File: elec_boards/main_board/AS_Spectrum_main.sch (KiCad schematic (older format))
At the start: 55 parts, among them J1 MODE, J10 Morpho_Gauche, J11 RN42X-DROITE, J12 POW-5V, J13 Bande1, J14 Morpho_Droite, J15 Lidar, J16 Bande2, J17 Bande3, J18 GND_reg, J19 Bande4, J2 POT_LUM, J20 Bande4.5, J21 Bande5, J22 nRF24L01, J23 Bande6, J24 Jack_Micro, J25 POT_AUDIO_10k, J3 COLORS, J32 LED Strip 1, J4 MISC, J5 POW_+12V, J6 Micro, J7 Jack, J8 POW-12V, J9 RN42X-GAUCHE

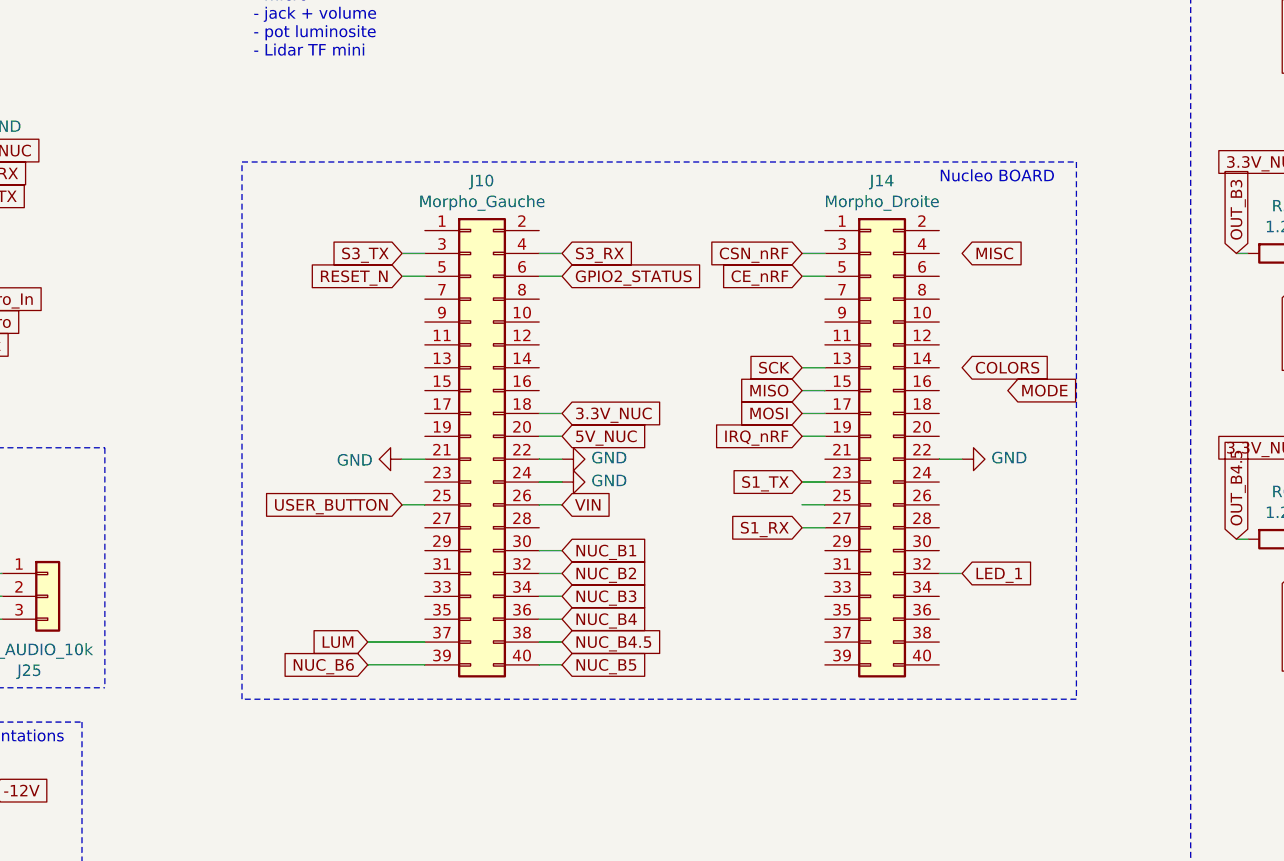
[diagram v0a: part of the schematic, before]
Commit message: Update Main Board Schematic and PCB
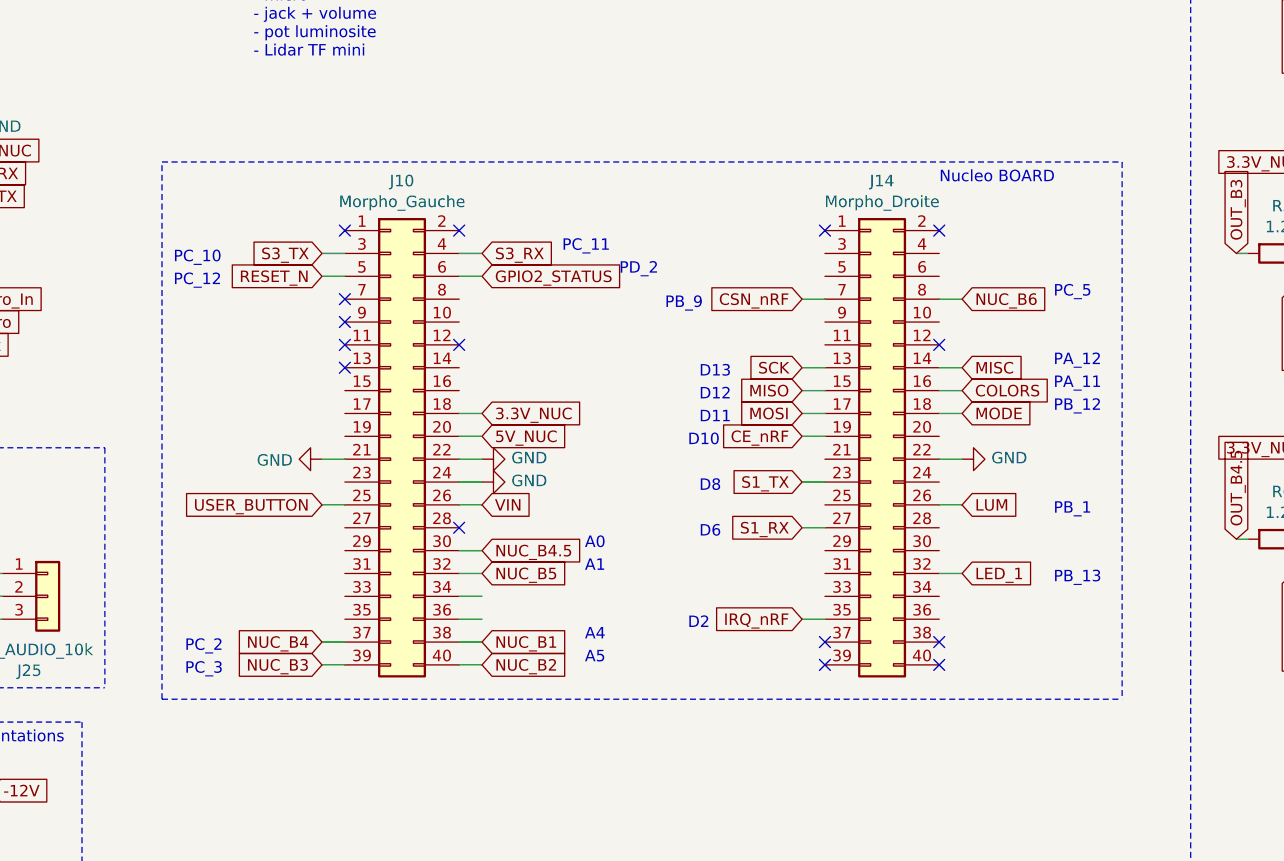
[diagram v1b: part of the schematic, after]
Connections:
- net CE_nRF: now also J14.19 (Pin_19); no longer J14.5 (Pin_5)
- net COLORS: now also J14.16 (Pin_16)
- net CSN_nRF: now also J14.7 (Pin_7); no longer J14.3 (Pin_3)
- net IRQ_nRF: now also J14.35 (Pin_35); no longer J14.19 (Pin_19)
- net LUM: now also J14.26 (Pin_26); no longer J10.37 (Pin_37)
- net MISC: now also J14.14 (Pin_14)
- net MODE: now also J14.18 (Pin_18)
- net NUC_B1: now also J10.38 (Pin_38); no longer J10.30 (Pin_30)
- net NUC_B2: now also J10.40 (Pin_40); no longer J10.32 (Pin_32)
- net NUC_B3: now also J10.39 (Pin_39); no longer J10.34 (Pin_34)
- net NUC_B4: now also J10.37 (Pin_37); no longer J10.36 (Pin_36)
- net NUC_B4.5: now also J10.30 (Pin_30); no longer J10.38 (Pin_38)
- net NUC_B5: now also J10.32 (Pin_32); no longer J10.40 (Pin_40)
- net NUC_B6: now also J14.8 (Pin_8); no longer J10.39 (Pin_39)
- no-connect marks 0 -> 15
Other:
- note added: "A0"
- note added: "A1"
- note added: "A4"
- note added: "A5"
- note added: "D10"
- note added: "D11"
- note added: "D12"
- note added: "D13"
- note added: "D2"
- note added: "D6"
- note added: "D8"
- note added: "PA_11"
- note added: "PA_12"
- note added: "PB_1"
- note added: "PB_12"
- note added: "PB_13"
- note added: "PB_9"
- note added: "PC_10"
- note added: "PC_11"
- note added: "PC_12"
- note added: "PC_2"
- note added: "PC_3"
- note added: "PC_5"
- note added: "PD_2"
- moved on the sheet: J10
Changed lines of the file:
@@
 L Connector_Generic:Conn_02x20_Odd_Even J10
 U 1 1 6028781C
-P 4600 3250
-F 0 "J10" H 4650 4367 50  0000 C CNN
-F 1 "Morpho_Gauche" H 4650 4276 50  0000 C CNN
-F 2 "Connector_PinHeader_2.54mm:PinHeader_2x20_P2.54mm_Vertical" H 4600 3250 50  0001 C CNN
-F 3 "~" H 4600 3250 50  0001 C CNN
-	1    4600 3250
+P 4250 3250
+F 0 "J10" H 4300 4367 50  0000 C CNN
+F 1 "Morpho_Gauche" H 4300 4276 50  0000 C CNN
+F 2 "Connector_PinHeader_2.54mm:PinHeader_2x20_P2.54mm_Vertical" H 4250 3250 50  0001 C CNN
+F 3 "~" H 4250 3250 50  0001 C CNN
+	1    4250 3250
 	1    0    0    -1
 $EndComp
@@
 	1    0    0    -1
 $EndComp
-Text GLabel 4300 2450 0    50   Input ~ 0
+Text GLabel 3950 2450 0    50   Input ~ 0
 S3_TX
 $Comp
 L power:GND #PWR02
 U 1 1 60290C89
-P 4300 3350
-F 0 "#PWR02" H 4300 3100 50  0001 C CNN
-F 1 "GND" V 4305 3222 50  0000 R CNN
-F 2 "" H 4300 3350 50  0001 C CNN
-F 3 "" H 4300 3350 50  0001 C CNN
-	1    4300 3350
+P 3950 3350
+F 0 "#PWR02" H 3950 3100 50  0001 C CNN
+F 1 "GND" V 3955 3222 50  0000 R CNN
+F 2 "" H 3950 3350 50  0001 C CNN
+F 3 "" H 3950 3350 50  0001 C CNN
+	1    3950 3350
 	0    1    1    0
 $EndComp
@@
 L power:GND #PWR03
 U 1 1 602916F0
-P 5000 3350
-F 0 "#PWR03" H 5000 3100 50  0001 C CNN
-F 1 "GND" V 5005 3222 50  0000 R CNN
-F 2 "" H 5000 3350 50  0001 C CNN
-F 3 "" H 5000 3350 50  0001 C CNN
-	1    5000 3350
+P 4650 3350
+F 0 "#PWR03" H 4650 3100 50  0001 C CNN
+F 1 "GND" V 4655 3222 50  0000 R CNN
+F 2 "" H 4650 3350 50  0001 C CNN
+F 3 "" H 4650 3350 50  0001 C CNN
+	1    4650 3350
 	0    -1   -1   0
 $EndComp
@@
 L power:GND #PWR04
 U 1 1 60291C87
-P 5000 3450
-F 0 "#PWR04" H 5000 3200 50  0001 C CNN
-F 1 "GND" V 5005 3322 50  0000 R CNN
-F 2 "" H 5000 3450 50  0001 C CNN
-F 3 "" H 5000 3450 50  0001 C CNN
-	1    5000 3450
+P 4650 3450
+F 0 "#PWR04" H 4650 3200 50  0001 C CNN
+F 1 "GND" V 4655 3322 50  0000 R CNN
+F 2 "" H 4650 3450 50  0001 C CNN
+F 3 "" H 4650 3450 50  0001 C CNN
+	1    4650 3450
 	0    -1   -1   0
 $EndComp
-Text GLabel 5000 3550 2    50   Input ~ 0
+Text GLabel 4650 3550 2    50   Input ~ 0
 VIN
-Text GLabel 5000 2450 2    50   Input ~ 0
+Text GLabel 4650 2450 2    50   Input ~ 0
 S3_RX
-Text GLabel 5000 3250 2    50   Input ~ 0
+Text GLabel 4650 3250 2    50   Input ~ 0
 5V_NUC
 Wire Wire Line
@@
 	6650 3350 6750 3350
 Wire Wire Line
-	5000 3250 4900 3250
-Wire Wire Line
-	4400 2450 4300 2450
-Wire Wire Line
-	4900 2450 5000 2450
-Wire Wire Line
-	4900 3350 5000 3350
-Wire Wire Line
-	4300 3350 4400 3350
-Wire Wire Line
-	4900 3450 5000 3450
-Wire Wire Line
-	4900 3550 5000 3550
+	4650 3250 4550 3250
+Wire Wire Line
+	4050 2450 3950 2450
+Wire Wire Line
+	4550 2450 4650 2450
+Wire Wire Line
+	4550 3350 4650 3350
+Wire Wire Line
+	3950 3350 4050 3350
+Wire Wire Line
+	4550 3450 4650 3450
+Wire Wire Line
+	4550 3550 4650 3550
 Wire Notes Line
 	4500 6350 6750 6350
@@
 RN42_MODULE
 Wire Notes Line
-	3600 2050 7250 2050
-Wire Notes Line
-	7250 2050 7250 4400
-Wire Notes Line
-	7250 4400 3600 4400
-Wire Notes Line
-	3600 4400 3600 2050
+	3250 4400 3250 2050
 Text Notes 6650 2150 0    50   ~ 0
 Nucleo BOARD
-Text GLabel 5000 2550 2    50   Input ~ 0
+Text GLabel 4650 2550 2    50   Input ~ 0
 GPIO2_STATUS
 Wire Wire Line
-	4900 2550 5000 2550
+	4550 2550 4650 2550
 $Comp
 L Connector_Generic:Conn_01x03 J18
@@
 Wire Wire Line
 	1050 6700 950  6700
-Text GLabel 5000 3150 2    50   Input ~ 0
+Text GLabel 4650 3150 2    50   Input ~ 0
 3.3V_NUC
 $Comp
@@
 	6400 7050 6500 7050
 Wire Wire Line
-	4900 3150 5000 3150
+	4550 3150 4650 3150
 $Comp
 L Connector_Generic:Conn_02x04_Odd_Even J22
@@
 Text GLabel 6050 3150 0    50   Input ~ 0
 MOSI
-Text GLabel 6050 3250 0    50   Input ~ 0
+Text GLabel 6050 4050 0    50   Input ~ 0
 IRQ_nRF
 Wire Wire Line
@@
 Wire Wire Line
 	6050 3450 6150 3450
-Wire Wire Line
-	6050 3550 6150 3550
 $Comp
 L power:GND #PWR0101
@@
 $EndComp
 Wire Wire Line
-	4900 3950 5000 3950
+	4550 3950 4650 3950
 $Comp
 L Connector_Generic:Conn_01x02 J5
@@
 Wire Wire Line
 	2150 6000 2250 6000
-Text GLabel 4300 3550 0    50   Input ~ 0
+Text GLabel 3950 3550 0    50   Input ~ 0
 USER_BUTTON
 Wire Wire Line
-	4300 3550 4400 3550
+	3950 3550 4050 3550
 Text Notes 3650 1600 0    50   ~ 0
 - Alim +/- 12V\n- ON/OFF\n- LED On/Off ( 3 alims - 12/-5/+5 )\n- switch MODE\n- switch COLOR\n- switch AUTRE\n- 7 bandes + limite 3.3V (Diode)\n- micro\n- jack + volume\n- pot luminosite\n- Lidar TF mini\n
@@
 	8300 1250 8300 1150
 Connection ~ 8300 1150
-Text GLabel 5000 3750 2    50   Input ~ 0
+Text GLabel 4650 4150 2    50   Input ~ 0
 NUC_B1
-Text GLabel 5000 3850 2    50   Input ~ 0
+Text GLabel 4650 4250 2    50   Input ~ 0
 NUC_B2
-Text GLabel 5000 3950 2    50   Input ~ 0
+Text GLabel 3950 4250 0    50   Input ~ 0
 NUC_B3
-Text GLabel 5000 4050 2    50   Input ~ 0
+Text GLabel 3950 4150 0    50   Input ~ 0
 NUC_B4
-Text GLabel 5000 4150 2    50   Input ~ 0
+Text GLabel 4650 3750 2    50   Input ~ 0
 NUC_B4.5
-Text GLabel 5000 4250 2    50   Input ~ 0
+Text GLabel 4650 3850 2    50   Input ~ 0
 NUC_B5
 Text GLabel 6050 3650 0    50   Input ~ 0
@@
 Wire Wire Line
 	2250 2200 2350 2200
-Text GLabel 4150 4250 0    50   Input ~ 0
+Text GLabel 6750 2650 2    50   Input ~ 0
 NUC_B6
 Wire Wire Line
-	4900 3750 5000 3750
-Wire Wire Line
-	4900 3850 5000 3850
-Wire Wire Line
-	4900 4050 5000 4050
-Wire Wire Line
-	4900 4150 5000 4150
-Wire Wire Line
-	4900 4250 5000 4250
-Wire Wire Line
-	4150 4250 4400 4250
-Text GLabel 4150 4150 0    50   Input ~ 0
-LUM
-Wire Wire Line
-	4150 4150 4400 4150
-Text GLabel 4300 2550 0    50   Input ~ 0
+	4550 3750 4650 3750
+Wire Wire Line
+	4550 3850 4650 3850
+Wire Wire Line
+	4550 4050 4650 4050
+Wire Wire Line
+	4550 4150 4650 4150
+Wire Wire Line
+	4550 4250 4650 4250
+Text GLabel 3950 2550 0    50   Input ~ 0
 RESET_N
 Wire Wire Line
-	4400 2550 4300 2550
-Text GLabel 6750 2450 2    50   Input ~ 0
+	4050 2550 3950 2550
+Text GLabel 6750 2950 2    50   Input ~ 0
 MISC
 Text GLabel 1850 4700 2    50   Input ~ 0
@@
 Wire Wire Line
 	6050 3250 6150 3250
-Text GLabel 6050 2450 0    50   Input ~ 0
-CSN_nRF
-Wire Wire Line
-	6050 2450 6150 2450
-Text GLabel 6050 2550 0    50   Input ~ 0
-CE_nRF
-Wire Wire Line
-	6050 2550 6150 2550
 $Comp
 L Device:CP C5
@@
 Wire Wire Line
 	6650 3850 6750 3850
-Text GLabel 6750 2950 2    50   Input ~ 0
+Text GLabel 6750 3050 2    50   Input ~ 0
 COLORS
-Text GLabel 6950 3050 2    50   Input ~ 0
+Text GLabel 6750 3150 2    50   Input ~ 0
 MODE
+Wire Wire Line
+	6750 2950 6650 2950
+Wire Wire Line
+	6750 3150 6650 3150
+Text GLabel 6750 3550 2    50   Input ~ 0
+LUM
+Wire Wire Line
+	6650 3550 6750 3550
+Wire Wire Line
+	6750 2650 6650 2650
+Text Notes 7150 2650 0    50   ~ 0
+PC_5
+Wire Wire Line
+	6650 3050 6750 3050
+Wire Wire Line
+	3950 4150 4050 4150
+Wire Wire Line
+	4050 4250 3950 4250
+Text Notes 5100 3750 0    50   ~ 0
+A0
+Text Notes 5100 3850 0    50   ~ 0
+A1
+Text Notes 5100 4150 0    50   ~ 0
+A4
+Text Notes 5100 4250 0    50   ~ 0
+A5
+Text Notes 3350 4300 0    50   ~ 0
+PC_3
+Text Notes 3350 4200 0    50   ~ 0
+PC_2
+Text Notes 7150 2950 0    50   ~ 0
+PA_12
+Text Notes 7150 3050 0    50   ~ 0
+PA_11
+Text Notes 7150 3150 0    50   ~ 0
+PB_12
+NoConn ~ 6150 2350
+NoConn ~ 6650 2350
+NoConn ~ 4050 2350
+NoConn ~ 4550 2350
+NoConn ~ 6650 2850
+NoConn ~ 6150 4250
+NoConn ~ 6150 4150
+NoConn ~ 6650 4150
+NoConn ~ 6650 4250
+NoConn ~ 4550 3650
+NoConn ~ 4550 2850
+NoConn ~ 4050 2850
+NoConn ~ 4050 2950
+NoConn ~ 4050 2650
+NoConn ~ 4050 2750
+Text Notes 5600 3000 0    50   ~ 0
+D13
+Text Notes 5600 3100 0    50   ~ 0
+D12
+Text Notes 5600 3200 0    50   ~ 0
+D11
+Text Notes 5550 4100 0    50   ~ 0
+D2
+Text Notes 5600 3500 0    50   ~ 0
+D8
+Text Notes 5600 3700 0    50   ~ 0
+D6
+Text Notes 3300 2500 0    50   ~ 0
+PC_10
+Text Notes 3300 2600 0    50   ~ 0
+PC_12
+Text Notes 5000 2450 0    50   ~ 0
+PC_11
+Text Notes 5250 2550 0    50   ~ 0
+PD_2
+Wire Notes Line
+	3250 2050 7450 2050
+Wire Notes Line
+	7450 2050 7450 4400
+Wire Notes Line
+	3250 4400 7450 4400
+Text Notes 7150 3900 0    50   ~ 0
+PB_13
+Text Notes 7150 3600 0    50   ~ 0
+PB_1
+Text GLabel 6050 2650 0    50   Input ~ 0
+CSN_nRF
+Wire Wire Line
+	6050 2650 6150 2650
+Text Notes 5450 2700 0    50   ~ 0
+PB_9
+Wire Wire Line
+	6050 4050 6150 4050
+Text Notes 5550 3300 0    50   ~ 0
+D10
+Text GLabel 6050 3250 0    50   Input ~ 0
+CE_nRF
 $EndSCHEMATC
